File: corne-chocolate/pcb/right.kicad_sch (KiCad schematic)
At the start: 79 parts, among them J3 MJ-4PP-9, J4 Conn_01x04, P3 Conn_01x01, P4 Conn_01x01, SW13 SW_PUSH, SW22 SW_PUSH, SW23 SW_PUSH, SW24 SW_PUSH, SW25 SW_PUSH, SW26 SW_PUSH, SW27 SW_PUSH, SW28 SW_PUSH, SW29 SW_PUSH, SW30 SW_PUSH, SW31 SW_PUSH, SW32 SW_PUSH, SW33 SW_PUSH, SW34 SW_PUSH, SW35 SW_PUSH, SW36 SW_PUSH, SW37 SW_PUSH, SW7 SW_PUSH, U2 ProMicro

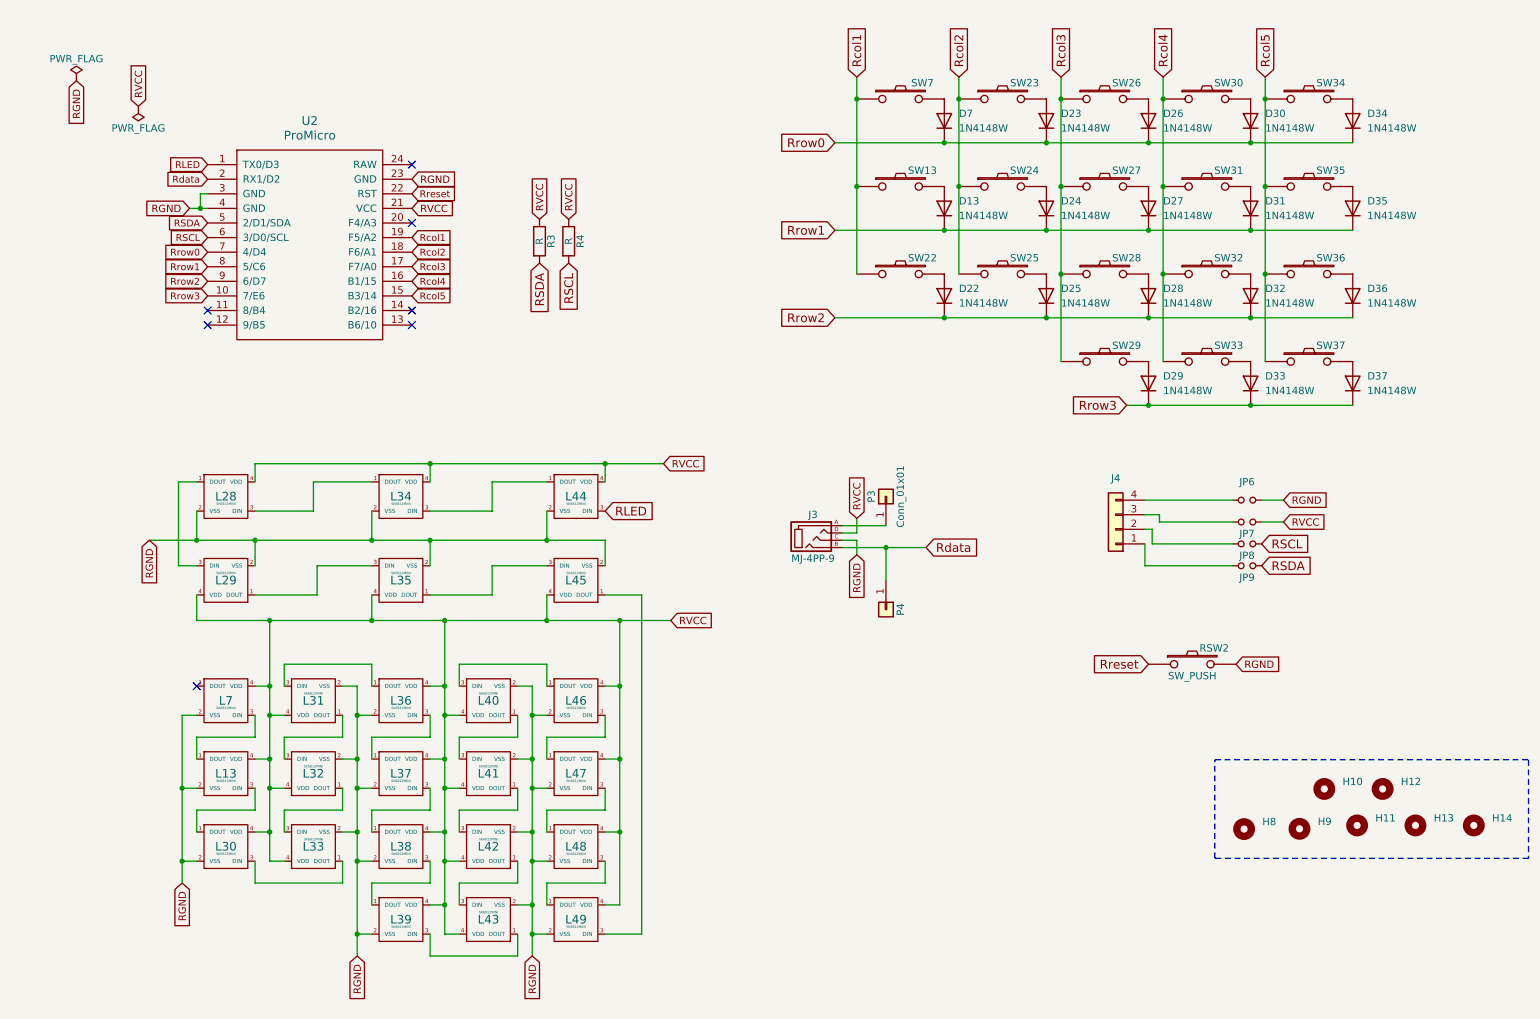
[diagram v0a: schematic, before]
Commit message: several important fixes
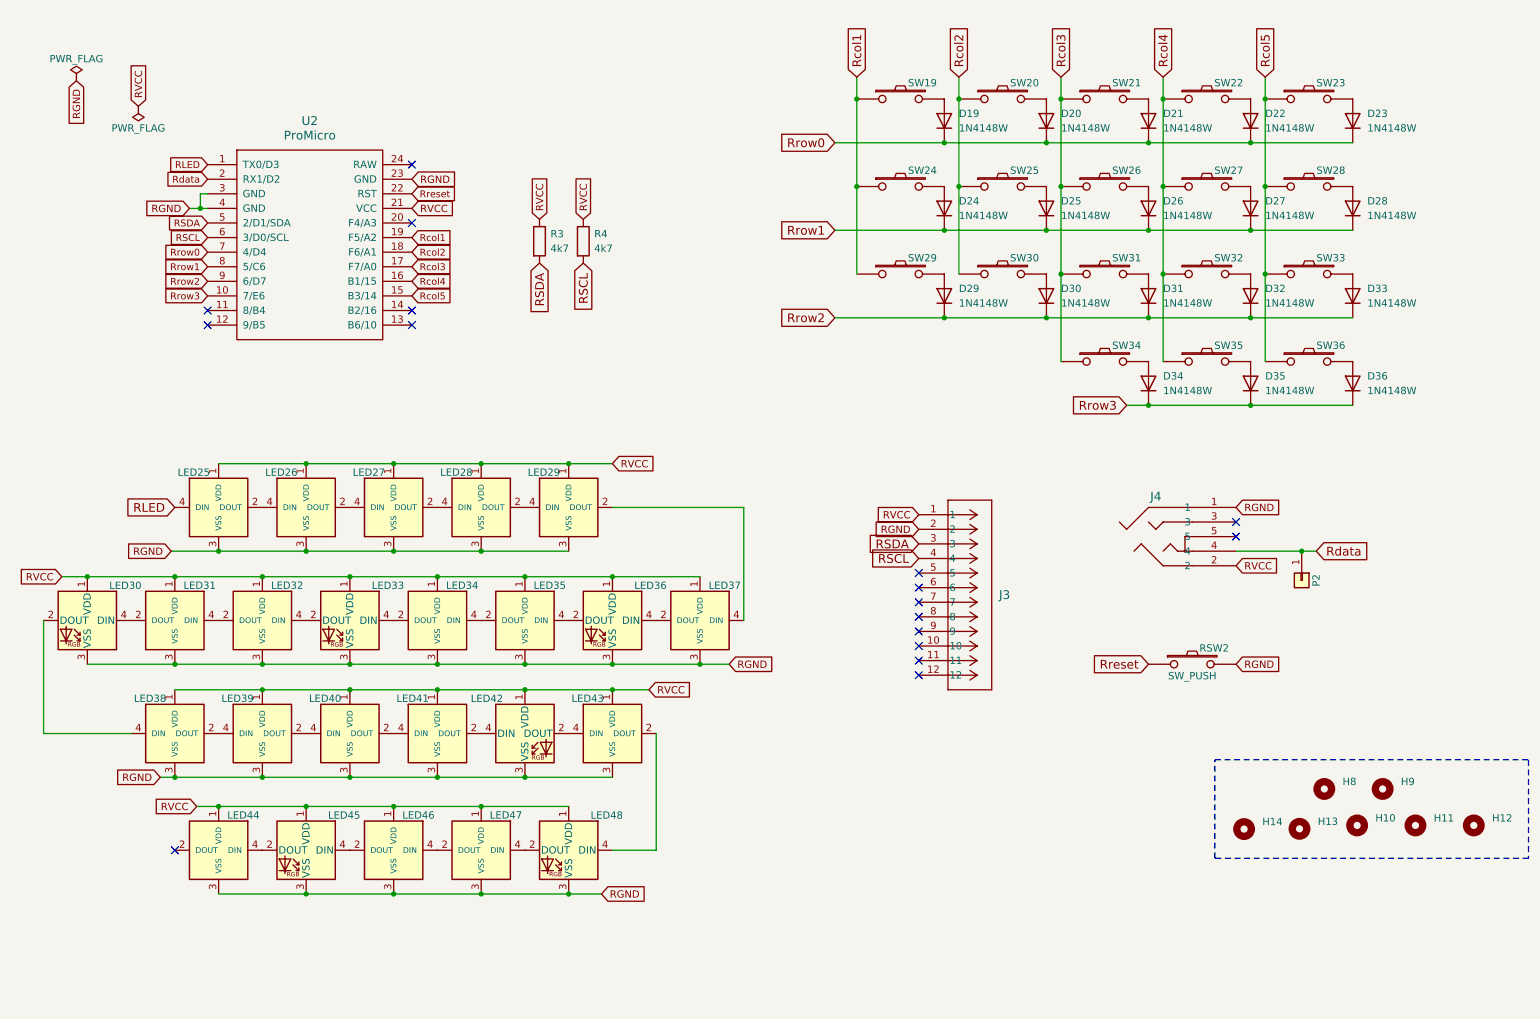
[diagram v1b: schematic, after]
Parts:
- removed J3: MJ-4PP-9, kbd:MJ-4PP-9_1side, symbol kbd:MJ-4PP-9
- removed J4: Conn_01x04, kbd:OLED_1side, symbol Connector_Generic:Conn_01x04
- removed JP6, JP7, JP8, JP9: Device:Jumper_NO_Small, kbd:Jumper, symbol kbd:Jumper_NO_Small-Device
- removed L13, L30, L31, L32, L33, L36, L37, L38, L39, L40, L41, L42, L43, L46, L47, L48, L49, L7: SK6812MINI, kbd:YS-SK6812MINI-E, symbol kbd:SK6812MINI
- removed L28, L29, L34, L35, L44, L45: SK6812MINI, kbd:SK6812MINI_underglow_rev, symbol kbd:SK6812MINI
- removed P3: Conn_01x01, kbd:1pin_conn, symbol Connector_Generic:Conn_01x01
- removed R3, R4: R, kbd:R, symbol Device:R
- added J3: 781271220, kbd:CON_781271220, symbol kbd:781271220
- added J4: 54-00174, kbd:54-00174_TEN, symbol kbd:54-00174
- added LED25, LED26, LED27, LED28, LED29, LED31, LED32, LED34, LED35, LED37, LED38, LED39, LED40, LED41, LED43, LED44, LED46, LED47: YS-SK6812MINI-E, kbd:LED_SK6812-MINI-E, symbol kbd:LED_SK6812MINI-E
- added LED30, LED33, LED36, LED42, LED45, LED48: WS2812B, kbd:LED_WS2812B_PLCC4_5.0x5.0mm_P3.2mm, symbol kbd:WS2812B
- added R3, R4: 4k7, kbd:R_1206_3216Metric_Pad1.30x1.75mm_HandSolder, symbol kbd:R
- D19: renamed from D7; item qty 100 -> (none); supplier Amazon -> Digikey; supplier pn B09DR5KFXM -> 1655-1N4148WCT-ND; vendor site https://www.amazon.com/Adafruit-Industries-1N4148-SOD-123-D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 -> (none)
- D20: renamed from D23; item qty 100 -> (none); supplier Amazon -> Digikey; supplier pn B09DR5KFXM -> 1655-1N4148WCT-ND; vendor site https://www.amazon.com/Adafruit-Industries-1N4148-SOD-123-D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 -> (none)
- D21: renamed from D26; item qty 100 -> (none); supplier Amazon -> Digikey; supplier pn B09DR5KFXM -> 1655-1N4148WCT-ND; vendor site https://www.amazon.com/Adafruit-Industries-1N4148-SOD-123-D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 -> (none)
- D22: renamed from D30; item qty 100 -> (none); supplier Amazon -> Digikey; supplier pn B09DR5KFXM -> 1655-1N4148WCT-ND; vendor site https://www.amazon.com/Adafruit-Industries-1N4148-SOD-123-D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 -> (none)
- D23: renamed from D34; item qty 100 -> (none); supplier Amazon -> Digikey; supplier pn B09DR5KFXM -> 1655-1N4148WCT-ND; vendor site https://www.amazon.com/Adafruit-Industries-1N4148-SOD-123-D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 -> (none)
- D24: renamed from D13; item qty 100 -> (none); supplier Amazon -> Digikey; supplier pn B09DR5KFXM -> 1655-1N4148WCT-ND; vendor site https://www.amazon.com/Adafruit-Industries-1N4148-SOD-123-D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 -> (none)
- D25: renamed from D24; item qty 100 -> (none); supplier Amazon -> Digikey; supplier pn B09DR5KFXM -> 1655-1N4148WCT-ND; vendor site https://www.amazon.com/Adafruit-Industries-1N4148-SOD-123-D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 -> (none)
- D26: renamed from D27; item qty 100 -> (none); supplier Amazon -> Digikey; supplier pn B09DR5KFXM -> 1655-1N4148WCT-ND; vendor site https://www.amazon.com/Adafruit-Industries-1N4148-SOD-123-D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 -> (none)
- D27: renamed from D31; item qty 100 -> (none); supplier Amazon -> Digikey; supplier pn B09DR5KFXM -> 1655-1N4148WCT-ND; vendor site https://www.amazon.com/Adafruit-Industries-1N4148-SOD-123-D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 -> (none)
- D28: renamed from D35; item qty 100 -> (none); supplier Amazon -> Digikey; supplier pn B09DR5KFXM -> 1655-1N4148WCT-ND; vendor site https://www.amazon.com/Adafruit-Industries-1N4148-SOD-123-D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 -> (none)
- D29: renamed from D22; item qty 100 -> (none); supplier Amazon -> Digikey; supplier pn B09DR5KFXM -> 1655-1N4148WCT-ND; vendor site https://www.amazon.com/Adafruit-Industries-1N4148-SOD-123-D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 -> (none)
- D30: renamed from D25; item qty 100 -> (none); supplier Amazon -> Digikey; supplier pn B09DR5KFXM -> 1655-1N4148WCT-ND; vendor site https://www.amazon.com/Adafruit-Industries-1N4148-SOD-123-D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 -> (none)
- D31: renamed from D28; item qty 100 -> (none); supplier Amazon -> Digikey; supplier pn B09DR5KFXM -> 1655-1N4148WCT-ND; vendor site https://www.amazon.com/Adafruit-Industries-1N4148-SOD-123-D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 -> (none)
- D32: item qty 100 -> (none); supplier Amazon -> Digikey; supplier pn B09DR5KFXM -> 1655-1N4148WCT-ND; vendor site https://www.amazon.com/Adafruit-Industries-1N4148-SOD-123-D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 -> (none)
- D33: renamed from D36; item qty 100 -> (none); supplier Amazon -> Digikey; supplier pn B09DR5KFXM -> 1655-1N4148WCT-ND; vendor site https://www.amazon.com/Adafruit-Industries-1N4148-SOD-123-D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 -> (none)
- D34: renamed from D29; item qty 100 -> (none); supplier Amazon -> Digikey; supplier pn B09DR5KFXM -> 1655-1N4148WCT-ND; vendor site https://www.amazon.com/Adafruit-Industries-1N4148-SOD-123-D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 -> (none)
- D35: renamed from D33; item qty 100 -> (none); supplier Amazon -> Digikey; supplier pn B09DR5KFXM -> 1655-1N4148WCT-ND; vendor site https://www.amazon.com/Adafruit-Industries-1N4148-SOD-123-D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 -> (none)
- D36: renamed from D37; item qty 100 -> (none); supplier Amazon -> Digikey; supplier pn B09DR5KFXM -> 1655-1N4148WCT-ND; vendor site https://www.amazon.com/Adafruit-Industries-1N4148-SOD-123-D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 -> (none)
- RSW2: item qty 50 -> (none); supplier Amazon -> Digikey; supplier 2 pn (none) -> B07H9ZSZD4; supplier pn B07H9ZSZD4 -> CKN12301-ND; supplier2 (none) -> Amazon; vendor site https://www.amazon.com/-/es/uxcell-0-118x0-236x0-197-Peque%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 -> (none)
- SW19: renamed from SW7; item qty 100 -> (none); supplier Amazon -> Digikey; supplier 2 pn (none) -> B0CPVJLMDJ; supplier pn B0CPVJLMDJ -> 1528-5118-ND; supplier2 (none) -> Amazon; vendor site https://www.amazon.com/100Pieces-Chocolate-Switches-Accesso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 -> (none)
- SW20: renamed from SW23; item qty 100 -> (none); supplier Amazon -> Digikey; supplier 2 pn (none) -> B0CPVJLMDJ; supplier pn B0CPVJLMDJ -> 1528-5118-ND; supplier2 (none) -> Amazon; vendor site https://www.amazon.com/100Pieces-Chocolate-Switches-Accesso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 -> (none)
- SW21: renamed from SW26; item qty 100 -> (none); supplier Amazon -> Digikey; supplier 2 pn (none) -> B0CPVJLMDJ; supplier pn B0CPVJLMDJ -> 1528-5118-ND; supplier2 (none) -> Amazon; vendor site https://www.amazon.com/100Pieces-Chocolate-Switches-Accesso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 -> (none)
- SW22: renamed from SW30; item qty 100 -> (none); supplier Amazon -> Digikey; supplier 2 pn (none) -> B0CPVJLMDJ; supplier pn B0CPVJLMDJ -> 1528-5118-ND; supplier2 (none) -> Amazon; vendor site https://www.amazon.com/100Pieces-Chocolate-Switches-Accesso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 -> (none)
- SW23: renamed from SW34; item qty 100 -> (none); supplier Amazon -> Digikey; supplier 2 pn (none) -> B0CPVJLMDJ; supplier pn B0CPVJLMDJ -> 1528-5118-ND; supplier2 (none) -> Amazon; vendor site https://www.amazon.com/100Pieces-Chocolate-Switches-Accesso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 -> (none)
- SW24: renamed from SW13; item qty 100 -> (none); supplier Amazon -> Digikey; supplier 2 pn (none) -> B0CPVJLMDJ; supplier pn B0CPVJLMDJ -> 1528-5118-ND; supplier2 (none) -> Amazon; vendor site https://www.amazon.com/100Pieces-Chocolate-Switches-Accesso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 -> (none)
- SW25: renamed from SW24; item qty 100 -> (none); supplier Amazon -> Digikey; supplier 2 pn (none) -> B0CPVJLMDJ; supplier pn B0CPVJLMDJ -> 1528-5118-ND; supplier2 (none) -> Amazon; vendor site https://www.amazon.com/100Pieces-Chocolate-Switches-Accesso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 -> (none)
- SW26: renamed from SW27; item qty 100 -> (none); supplier Amazon -> Digikey; supplier 2 pn (none) -> B0CPVJLMDJ; supplier pn B0CPVJLMDJ -> 1528-5118-ND; supplier2 (none) -> Amazon; vendor site https://www.amazon.com/100Pieces-Chocolate-Switches-Accesso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 -> (none)
- SW27: renamed from SW31; item qty 100 -> (none); supplier Amazon -> Digikey; supplier 2 pn (none) -> B0CPVJLMDJ; supplier pn B0CPVJLMDJ -> 1528-5118-ND; supplier2 (none) -> Amazon; vendor site https://www.amazon.com/100Pieces-Chocolate-Switches-Accesso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 -> (none)
- SW28: renamed from SW35; item qty 100 -> (none); supplier Amazon -> Digikey; supplier 2 pn (none) -> B0CPVJLMDJ; supplier pn B0CPVJLMDJ -> 1528-5118-ND; supplier2 (none) -> Amazon; vendor site https://www.amazon.com/100Pieces-Chocolate-Switches-Accesso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 -> (none)
- SW29: renamed from SW22; item qty 100 -> (none); supplier Amazon -> Digikey; supplier 2 pn (none) -> B0CPVJLMDJ; supplier pn B0CPVJLMDJ -> 1528-5118-ND; supplier2 (none) -> Amazon; vendor site https://www.amazon.com/100Pieces-Chocolate-Switches-Accesso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 -> (none)
- SW30: renamed from SW25; item qty 100 -> (none); supplier Amazon -> Digikey; supplier 2 pn (none) -> B0CPVJLMDJ; supplier pn B0CPVJLMDJ -> 1528-5118-ND; supplier2 (none) -> Amazon; vendor site https://www.amazon.com/100Pieces-Chocolate-Switches-Accesso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 -> (none)
- SW31: renamed from SW28; item qty 100 -> (none); supplier Amazon -> Digikey; supplier 2 pn (none) -> B0CPVJLMDJ; supplier pn B0CPVJLMDJ -> 1528-5118-ND; supplier2 (none) -> Amazon; vendor site https://www.amazon.com/100Pieces-Chocolate-Switches-Accesso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 -> (none)
- SW32: item qty 100 -> (none); supplier Amazon -> Digikey; supplier 2 pn (none) -> B0CPVJLMDJ; supplier pn B0CPVJLMDJ -> 1528-5118-ND; supplier2 (none) -> Amazon; vendor site https://www.amazon.com/100Pieces-Chocolate-Switches-Accesso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 -> (none)
- SW33: renamed from SW36; item qty 100 -> (none); supplier Amazon -> Digikey; supplier 2 pn (none) -> B0CPVJLMDJ; supplier pn B0CPVJLMDJ -> 1528-5118-ND; supplier2 (none) -> Amazon; vendor site https://www.amazon.com/100Pieces-Chocolate-Switches-Accesso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 -> (none)
- SW34: renamed from SW29; item qty 100 -> (none); supplier Amazon -> Digikey; supplier 2 pn (none) -> B0CPVJLMDJ; supplier pn B0CPVJLMDJ -> 1528-5118-ND; supplier2 (none) -> Amazon; vendor site https://www.amazon.com/100Pieces-Chocolate-Switches-Accesso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 -> (none)
- SW35: renamed from SW33; item qty 100 -> (none); supplier Amazon -> Digikey; supplier 2 pn (none) -> B0CPVJLMDJ; supplier pn B0CPVJLMDJ -> 1528-5118-ND; supplier2 (none) -> Amazon; vendor site https://www.amazon.com/100Pieces-Chocolate-Switches-Accesso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 -> (none)
- SW36: renamed from SW37; item qty 100 -> (none); supplier Amazon -> Digikey; supplier 2 pn (none) -> B0CPVJLMDJ; supplier pn B0CPVJLMDJ -> 1528-5118-ND; supplier2 (none) -> Amazon; vendor site https://www.amazon.com/100Pieces-Chocolate-Switches-Accesso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 -> (none)
- U2: supplier (none) -> Digikey; supplier 2 pn (none) -> B09TKMM8N5; supplier pn (none) -> 1568-1060-ND; supplier2 (none) -> Amazon
- renumbered H11 to H10, H13 to H11, H14 to H12, H9 to H13, H8 to H14, H10 to H8, H12 to H9, P4 to P2
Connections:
- net RGND: now also J3.2, J4.1, LED25.3 (VSS), LED26.3 (VSS), LED27.3 (VSS), LED28.3 (VSS), LED29.3 (VSS), LED30.3 (VSS), LED31.3 (VSS), LED32.3 (VSS), LED33.3 (VSS), LED34.3 (VSS), LED35.3 (VSS), LED36.3 (VSS), LED37.3 (VSS), LED38.3 (VSS), LED39.3 (VSS), LED40.3 (VSS), LED41.3 (VSS), LED42.3 (VSS), LED43.3 (VSS), LED44.3 (VSS), LED45.3 (VSS), LED46.3 (VSS), LED47.3 (VSS), LED48.3 (VSS)
- net RLED: now also LED25.4 (DIN)
- net RSCL: now also J3.4, R4.2
- net RSDA: now also J3.3, R3.2
- net RVCC: now also J3.1, J4.2, LED25.1 (VDD), LED26.1 (VDD), LED27.1 (VDD), LED28.1 (VDD), LED29.1 (VDD), LED30.1 (VDD), LED31.1 (VDD), LED32.1 (VDD), LED33.1 (VDD), LED34.1 (VDD), LED35.1 (VDD), LED36.1 (VDD), LED37.1 (VDD), LED38.1 (VDD), LED39.1 (VDD), LED40.1 (VDD), LED41.1 (VDD), LED42.1 (VDD), LED43.1 (VDD), LED44.1 (VDD), LED45.1 (VDD), LED46.1 (VDD), LED47.1 (VDD), LED48.1 (VDD), R3.1, R4.1
- net Rdata: now also J4.4
- new net: LED31.4 (DIN), LED32.2 (DOUT)
- new net: LED32.4 (DIN), LED33.2 (DOUT)
- new net: LED26.2 (DOUT), LED27.4 (DIN)
- new net: LED25.2 (DOUT), LED26.4 (DIN)
- new net: LED43.2 (DOUT), LED48.4 (DIN)
- new net: LED42.2 (DOUT), LED43.4 (DIN)
- new net: LED44.4 (DIN), LED45.2 (DOUT)
- new net: LED47.4 (DIN), LED48.2 (DOUT)
- new net: LED33.4 (DIN), LED34.2 (DOUT)
- new net: LED41.2 (DOUT), LED42.4 (DIN)
- new net: LED40.2 (DOUT), LED41.4 (DIN)
- new net: LED39.2 (DOUT), LED40.4 (DIN)
- new net: LED38.2 (DOUT), LED39.4 (DIN)
- new net: LED36.4 (DIN), LED37.2 (DOUT)
- new net: LED29.2 (DOUT), LED37.4 (DIN)
- new net: LED27.2 (DOUT), LED28.4 (DIN)
- new net: LED35.4 (DIN), LED36.2 (DOUT)
- new net: LED34.4 (DIN), LED35.2 (DOUT)
- new net: LED28.2 (DOUT), LED29.4 (DIN)
- new net: LED45.4 (DIN), LED46.2 (DOUT)
- new net: LED46.4 (DIN), LED47.2 (DOUT)
- new net: LED30.2 (DOUT), LED38.4 (DIN)
- new net: LED30.4 (DIN), LED31.2 (DOUT)
- no-connect marks 7 -> 17
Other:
- moved on the sheet: P2
